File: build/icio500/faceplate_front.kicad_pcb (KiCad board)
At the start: 4 copper layers, 38.1 x 133.3 mm, 3 parts

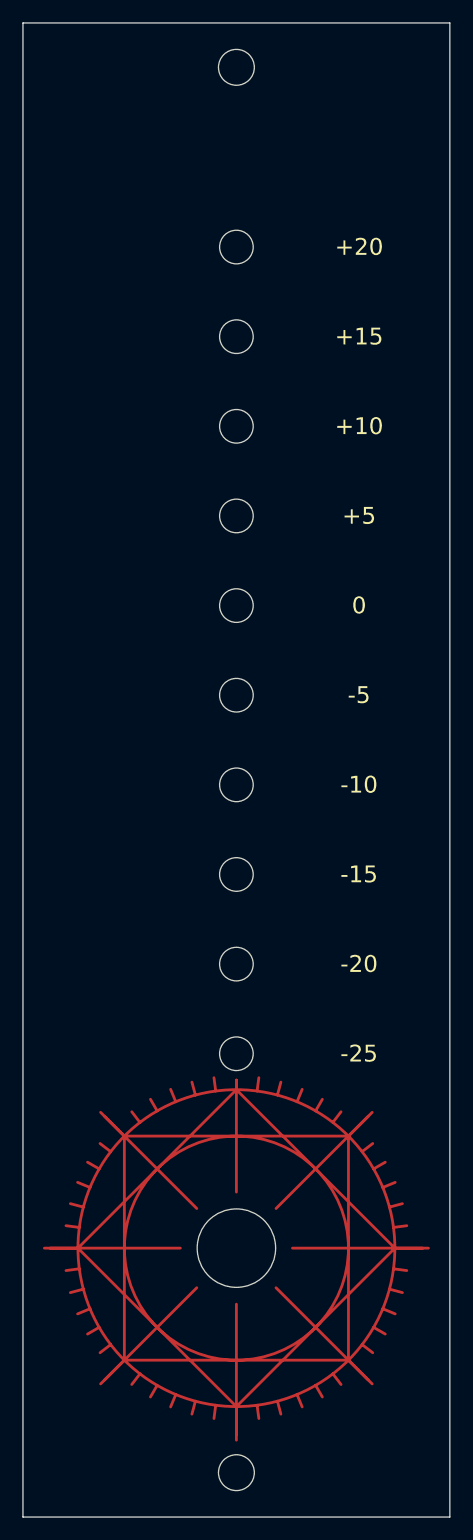
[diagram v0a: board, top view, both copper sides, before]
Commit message: Restore finished 10-27 faceplate & satellite; maintain summer VPR card edge with zero DRC violations
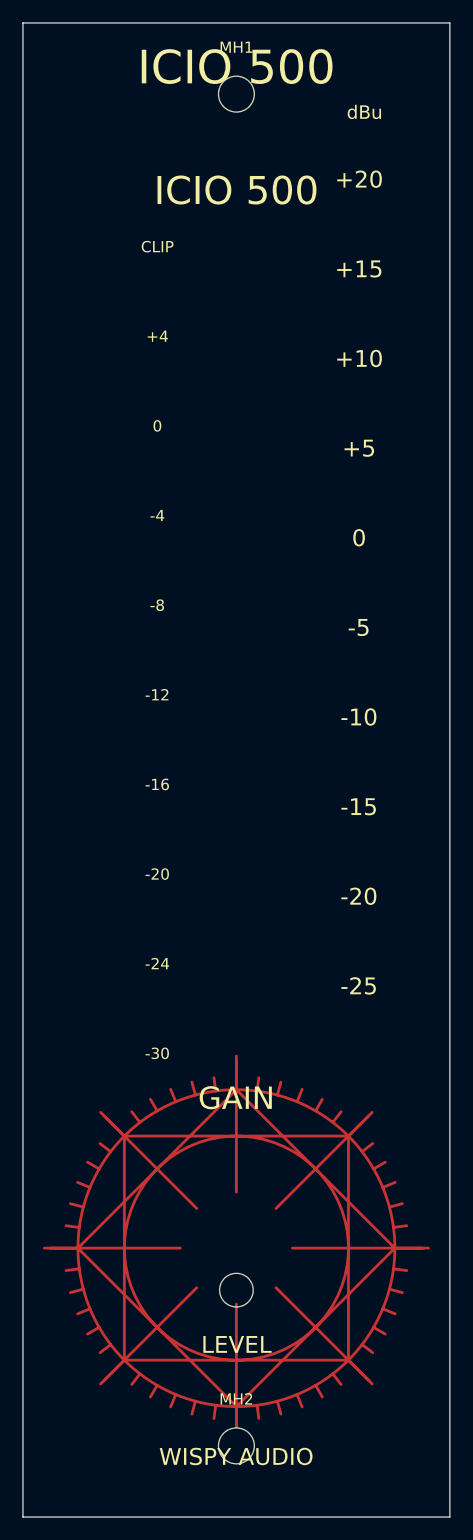
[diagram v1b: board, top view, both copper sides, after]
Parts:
- moved MH1 2.39 mm to (19.1, 6.35)
- moved MH2 2.39 mm to (19.1, 127.0)
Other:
- outline, holes or cut-outs redrawn
- board text added: "+4"
- board text added: "-12"
- board text added: "-16"
- board text added: "-24"
- board text added: "-30"
- board text added: "-4"
- board text added: "-8"
- board text added: "CLIP"
- board text added: "GAIN"
- board text added: "ICIO 500"
- board text added: "LEVEL"
- board text added: "WISPY AUDIO"
- board text added: "dBu"
